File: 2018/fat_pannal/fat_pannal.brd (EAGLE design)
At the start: 160 x 130.5 mm, 33 parts, among them IC1 MEGA8-P, Q2 BUZ11BV, Q3 BUZ11BV, Q4 BUZ11BV, Q5 BUZ11BV, U1 TSR_1-2450

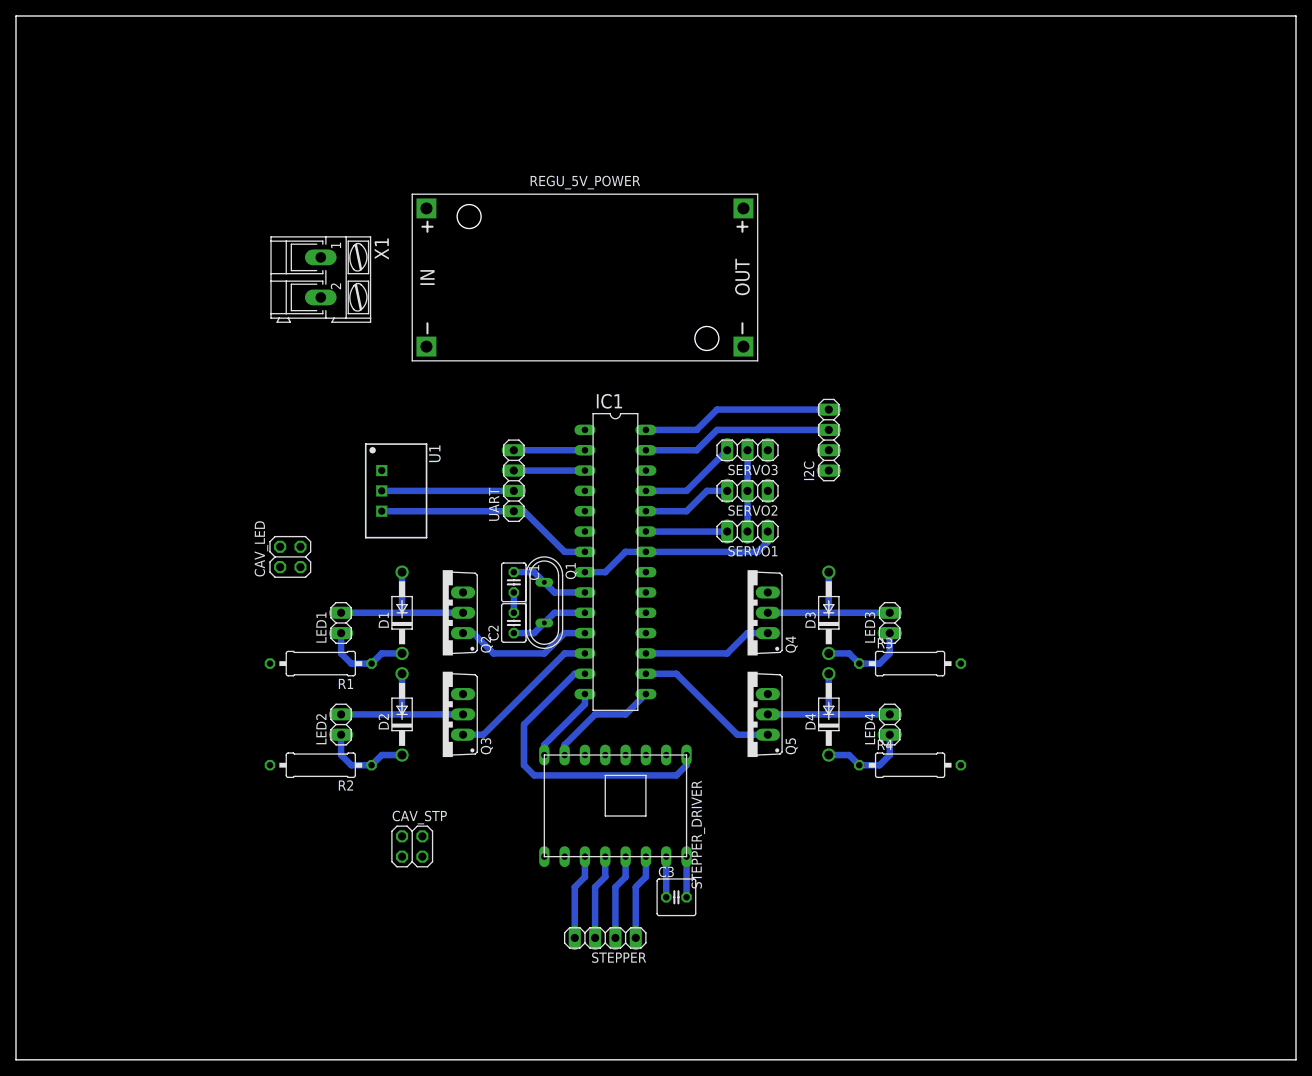
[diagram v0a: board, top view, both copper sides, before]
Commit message: [FAT pannal] Finish board V1.
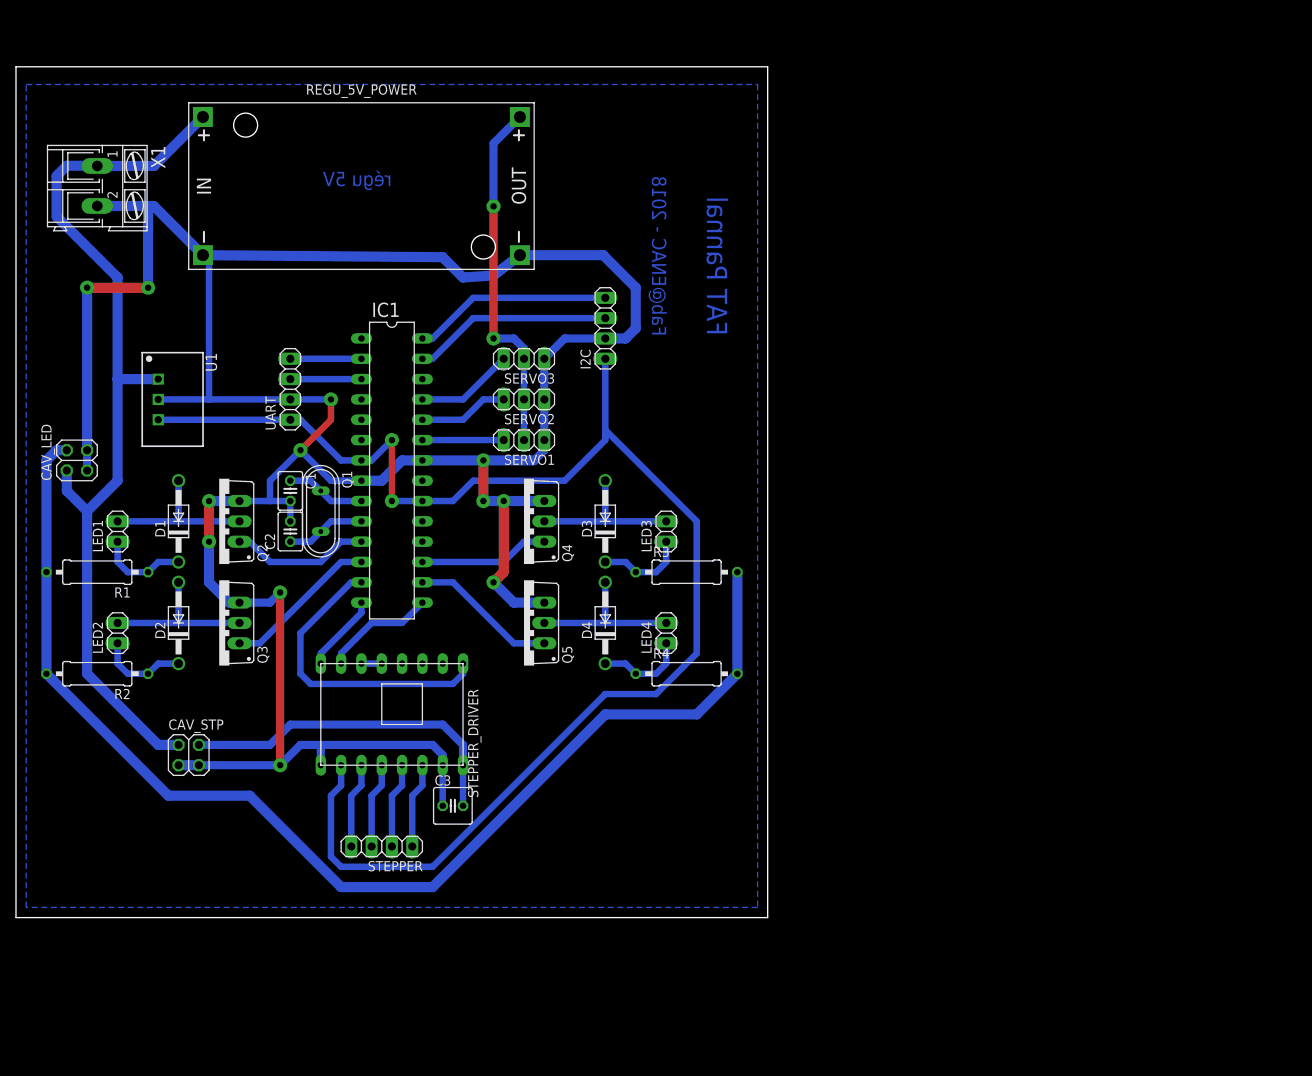
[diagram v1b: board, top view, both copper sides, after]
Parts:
- moved I2C 31.2 mm to (73.7, 73.7)
- moved R3 30.2 mm to (83.8, 43.2)
- moved R4 30.2 mm to (83.8, 30.5)
- moved CAV_STP 30.2 mm to (21.6, 20.3)
- moved IC1 30.2 mm to (47.0, 55.9)
- moved LED1 30.2 mm to (12.7, 48.3)
- moved LED2 30.2 mm to (12.7, 35.6)
- moved Q1 30.2 mm to (38.1, 50.8)
- moved Q2 30.2 mm to (25.4, 49.5)
- moved Q3 30.2 mm to (25.4, 36.8)
- moved R1 30.2 mm to (10.2, 43.2)
- moved R2 30.2 mm to (10.2, 30.5)
- moved REGU_5V_POWER 30.2 mm to (43.2, 91.4)
- moved STEPPER_DRIVER 30.2 mm to (48.3, 24.1)
- moved C1 30.2 mm to (34.3, 53.3)
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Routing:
- net GND: track 49.8 -> 363.0 mm, vias 0 -> 12
- net 5V_SIG: track 27.5 -> 181.9 mm, vias 0 -> 2
- net VLED: track 0.00 -> 150.9 mm
- net VBAT: track 0.00 -> 114.6 mm
- net VMOT: track 5.08 -> 42.7 mm
- net 5V_POWER: track 10.2 -> 44.8 mm, vias 0 -> 2
- net N$9: track 0.00 -> 2.54 mm
- net SDA: track 23.9 -> 25.0 mm
- net SCL: track 23.9 -> 25.0 mm
- added copper zone on layer 16, net GND
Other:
- board size 160 x 130.5 mm -> 94 x 106.3 mm
- board text added: "FAT Pannal"
- board text added: "Fab@ENAC - 2018"
- board text added: "régu 5V"
